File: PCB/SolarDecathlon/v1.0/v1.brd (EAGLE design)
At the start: 111.9 x 84.6 mm, 75 parts, among them CON1 SPI, IC1 REG1117, J1 RJ12, J2 RJ12, J3 RJ12, J4 RJ12, J5 RJ12, J6 RJ12, Q1 BSP75, Q2 BSP75, Q3 BSP75, Q4 BSP75, Q5 BSP75, Q6 BSP75, X3 16MHz, X4 MINI-USB

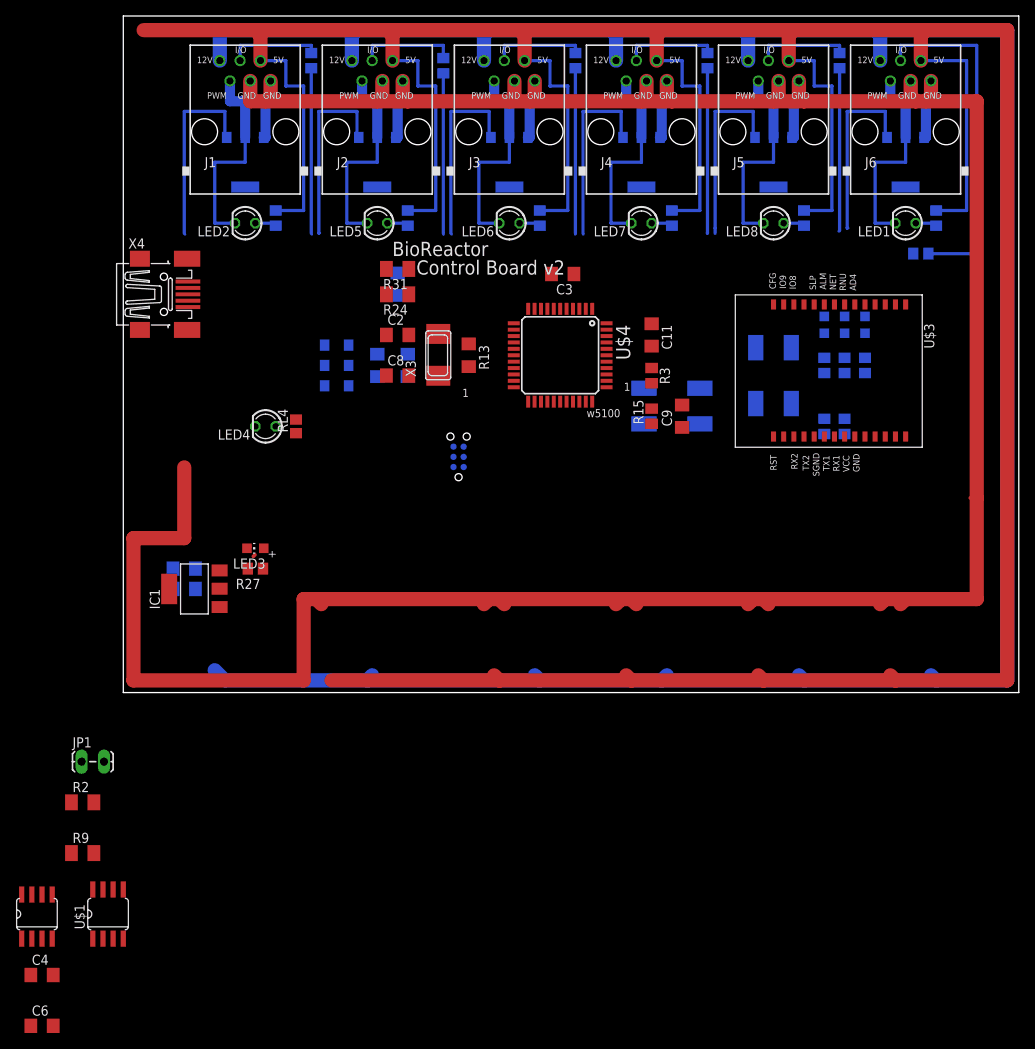
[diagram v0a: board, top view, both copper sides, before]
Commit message: Update wiegand
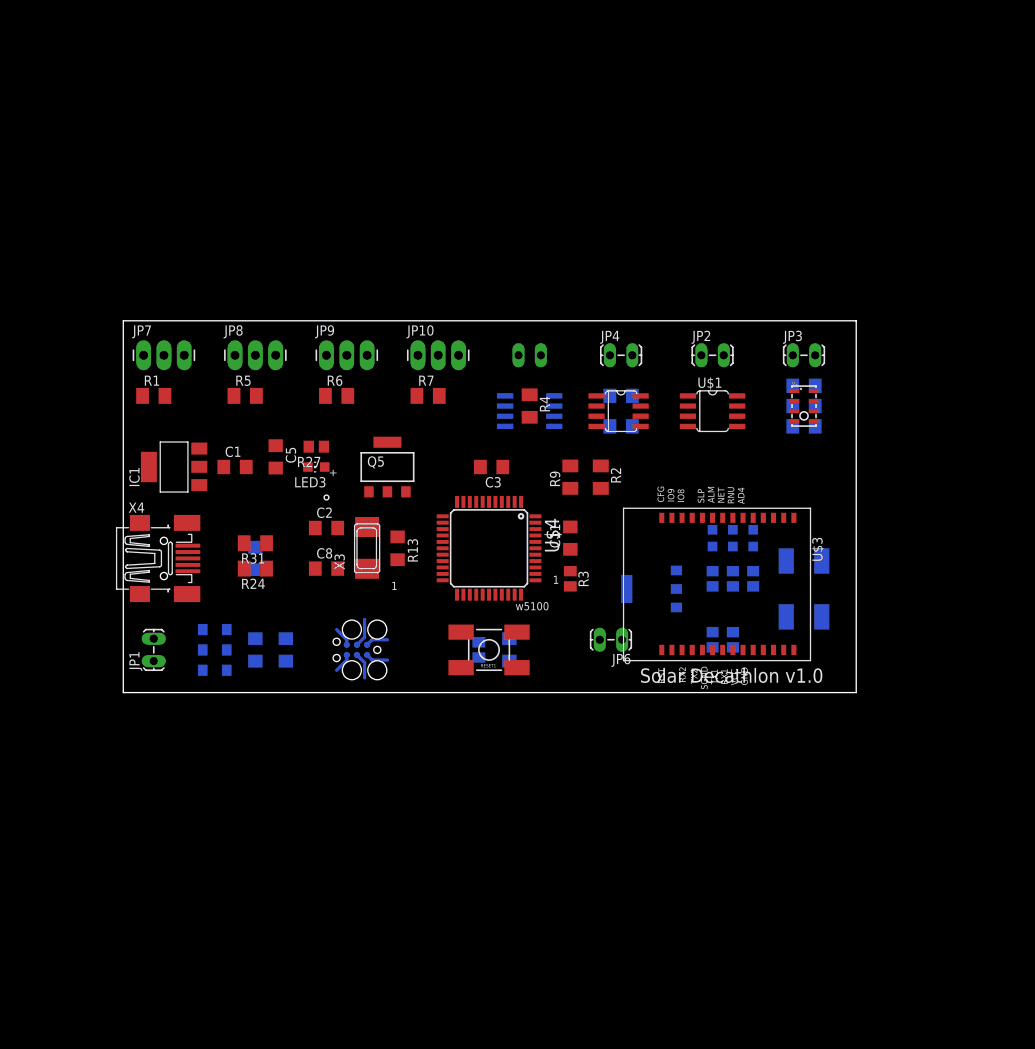
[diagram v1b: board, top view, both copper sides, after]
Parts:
- removed J1, J2, J3, J4, J5, J6: RJ12, lpatiny:RJ12-STRAIGHT
- removed LED1, LED2, LED5, LED6, LED8: Blue, lpatiny:LED3MM
- removed LED4: RED, lpatiny:LED3MM
- removed LED7: BLue, lpatiny:LED3MM
- removed Q1, Q2, Q4, Q6: BSP75, infineon:PG-SOT-223
- removed R, R19, R20, R25, R32, R33, R34, R35: 1k, rcl:R0805
- removed RL4: 1K, resistor:R0805
- added C13, C15: 100nF, rcl:C1206
- added C14: 10uF, rcl:C1206
- added JP10, JP7, JP8, JP9: (no value), SparkFun:1X03_LONGPADS
- added JP2, JP3, JP4, JP5, JP6: (no value), SparkFun:1X02_LOCK_LONGPADS
- added R1: 4.7k, resistor:M1206
- added U$5: DS18B20, lpatiny:SO8
- added U1: MPL3115A2LGA8, SparkFun-Sensors:LGA8
- CON1: device lpatiny:TC2030-MCP-NL -> lpatiny:TC2030-MCP
- R4, R5, R6, R7: value 1k -> 4.7k; device rcl:R0805 -> resistor:M1206
- moved C6 104.2 mm to (62.2, 30.5), flipped to the bottom, turned to 180 degrees
- moved C4 102.4 mm to (62.2, 34.3), flipped to the bottom, turned to 180 degrees
- moved U$1 95.6 mm to (73.7, 30.5), turned to 270 degrees
- moved U$2 95.5 mm to (62.2, 31.8), turned to 270 degrees
- moved R9 77.0 mm to (55.9, 24.1), turned to 90 degrees
- moved R2 76.5 mm to (59.7, 24.1), turned to 270 degrees
- moved Q3 62.1 mm to (66.0, 10.2), turned to 270 degrees
- moved R7 52.0 mm to (38.1, 34.3), flipped to the top, turned to 0 degrees
- moved Q5 49.6 mm to (33.0, 25.4), flipped to the top, turned to 0 degrees
- moved R6 47.4 mm to (26.7, 34.3), flipped to the top, turned to 0 degrees
- moved R5 43.0 mm to (15.2, 34.3), flipped to the top, turned to 0 degrees
- moved D2 41.0 mm to (11.4, 2.54)
- moved C10 38.7 mm to (16.5, 2.54)
- moved C12 38.7 mm to (20.3, 2.54)
- moved D3 38.7 mm to (11.4, 0.00)
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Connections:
- removed net +12V: J1.+12V, J2.+12V, J3.+12V, J4.+12V, J5.+12V, J6.+12V
- removed net N$1: J3.PWM, LED6.K, Q4.2
- removed net N$12: LED4.A, RL4.2
- removed net N$17: LED2.A, R25.1
- removed net N$18: J1.I/O, R.2
- removed net N$19: J5.PWM, LED8.K, Q6.2
- removed net N$21: J6.PWM, LED1.K, Q3.2
- removed net N$22: LED6.A, R5.1
- removed net N$28: J2.PWM, LED5.K, Q2.2
- removed net N$29: J4.I/O, R34.2
- removed net N$3: J6.I/O, R19.2
- removed net N$30: LED7.A, R6.1
- removed net N$32: J5.I/O, R35.2
- removed net N$33: LED8.A, R7.1
- removed net N$34: J1.PWM, LED2.K, Q1.2
- removed net N$4: LED5.A, R4.1
- removed net N$5: J4.PWM, LED7.K, Q5.2
- removed net N$7: J3.I/O, R33.2
- removed net N$9: LED1.A, R20.1
- new net $1: C13.2, C14.2, C15.2, JP3.1, U1.3
- new net $12: JP2.1, U$1.4
- new net $2: C4.2, C6.2, JP4.1, U$2.2
- new net $3: JP5.1, U$5.5
- new net GND_CONTROLLED: JP2.2, JP3.2, JP4.2, JP5.2, Q3.2, Q5.3
- new net N$13: C15.1, U1.2
- new net N$8: JP6.1, U$3.GND
- net +5V: no longer J1.+5V, J2.+5V, J3.+5V, J4.+5V, J5.+5V, J6.+5V, R20.2, R25.2, R4.2, R5.2, R6.2, R7.2
- net 3.3V: now also C13.1, C14.1, JP10.1, JP7.1, JP8.1, JP9.1, R1.1, R4.1, R5.1, R6.1, R7.1, U$5.3, U1.1, U1.4
- net A0: now also R4.2, U$5.4; no longer R35.1
- net A1: now also JP9.2, R6.2; no longer R33.1
- net A2: now also JP8.2, R5.2; no longer R32.1
- net A3: now also JP7.2, R1.2; no longer R.1
- net A4: now also JP10.2, R7.2; no longer R34.1
- net A5: no longer R19.1
- net D10*: no longer Q3.1
- net D11*: no longer Q6.1
- net D5*: no longer Q5.1
- net D6*: now also Q5.1; no longer Q1.1
- net D8*: now also Q3.1; no longer Q2.1
- net D9*: no longer Q4.1
- net GND: now also JP10.3, JP7.3, JP8.3, JP9.3; no longer C4.2, C6.2, J1.GND1, J1.GND2, J2.GND1, J2.GND2, J3.GND1, J3.GND2, J4.GND1, J4.GND2, J5.GND1, J5.GND2, J6.GND1, J6.GND2, LED4.K, Q1.3, Q2.3, Q4.3, Q5.3, Q6.3, U$1.4, U$2.2, U$3.GND
- net N$2: now also JP6.2, Q5.2; no longer J2.I/O, R32.2
- net SCL: now also U1.8
- net SDA: now also U1.7
- net VCC: no longer RL4.1
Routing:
- net +5V: track 468.1 -> 0.00 mm
- net GND: track 392.4 -> 2.43 mm
- net +12V: track 308.0 -> 0.00 mm
- net N$3: track 59.1 -> 0.00 mm
- net N$19: track 26.0 -> 0.00 mm
- net N$34: track 26.0 -> 0.00 mm
- net N$28: track 26.0 -> 0.00 mm
- net N$21: track 26.0 -> 0.00 mm
- net N$1: track 26.0 -> 0.00 mm
- net N$5: track 26.0 -> 0.00 mm
- net D6*: track 24.0 -> 0.00 mm
- net D9*: track 23.7 -> 0.00 mm
- net D5*: track 23.6 -> 0.00 mm
- net D8*: track 23.6 -> 0.00 mm
- net D11*: track 23.5 -> 0.00 mm
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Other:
- board size 111.9 x 84.6 mm -> 91.6 x 46.5 mm
- board text added: "Solar Decathlon v1.0"
- board text removed: "BioReactor"
- board text removed: "Control Board v2"

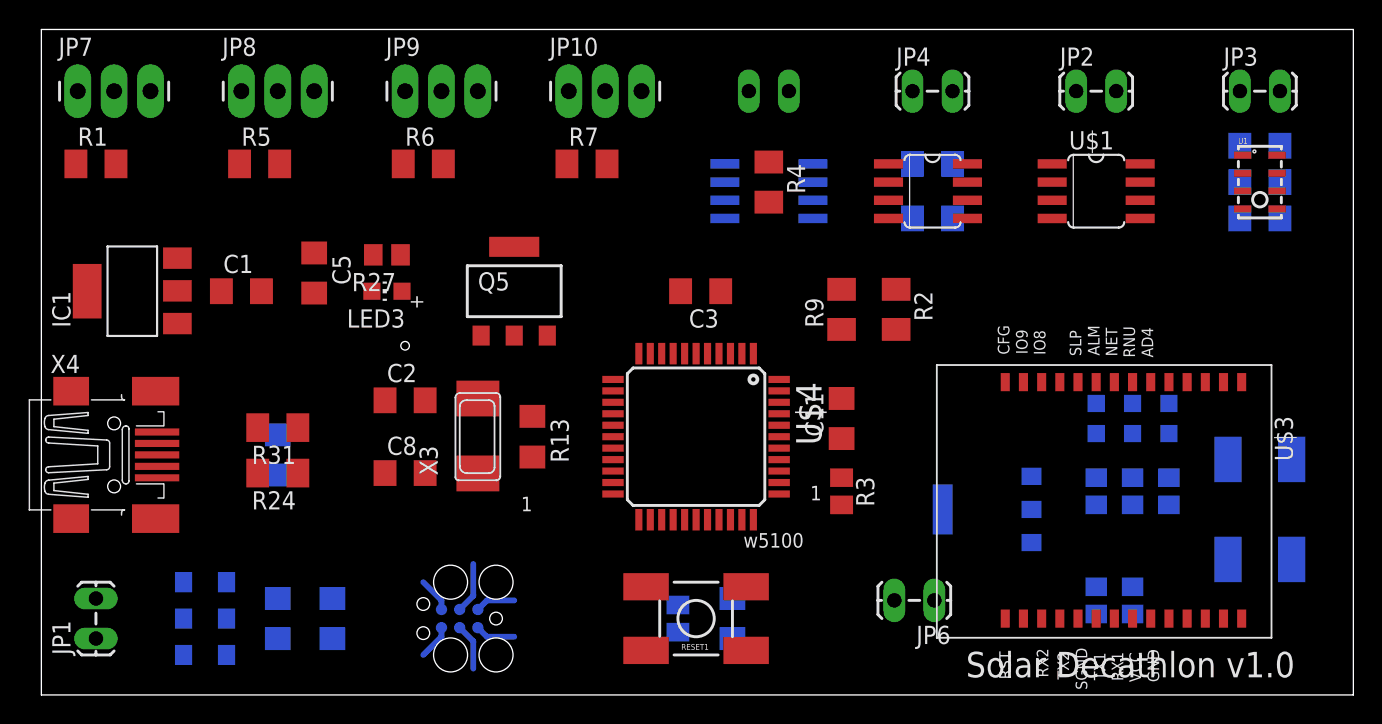
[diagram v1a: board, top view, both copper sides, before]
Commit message: Add routing
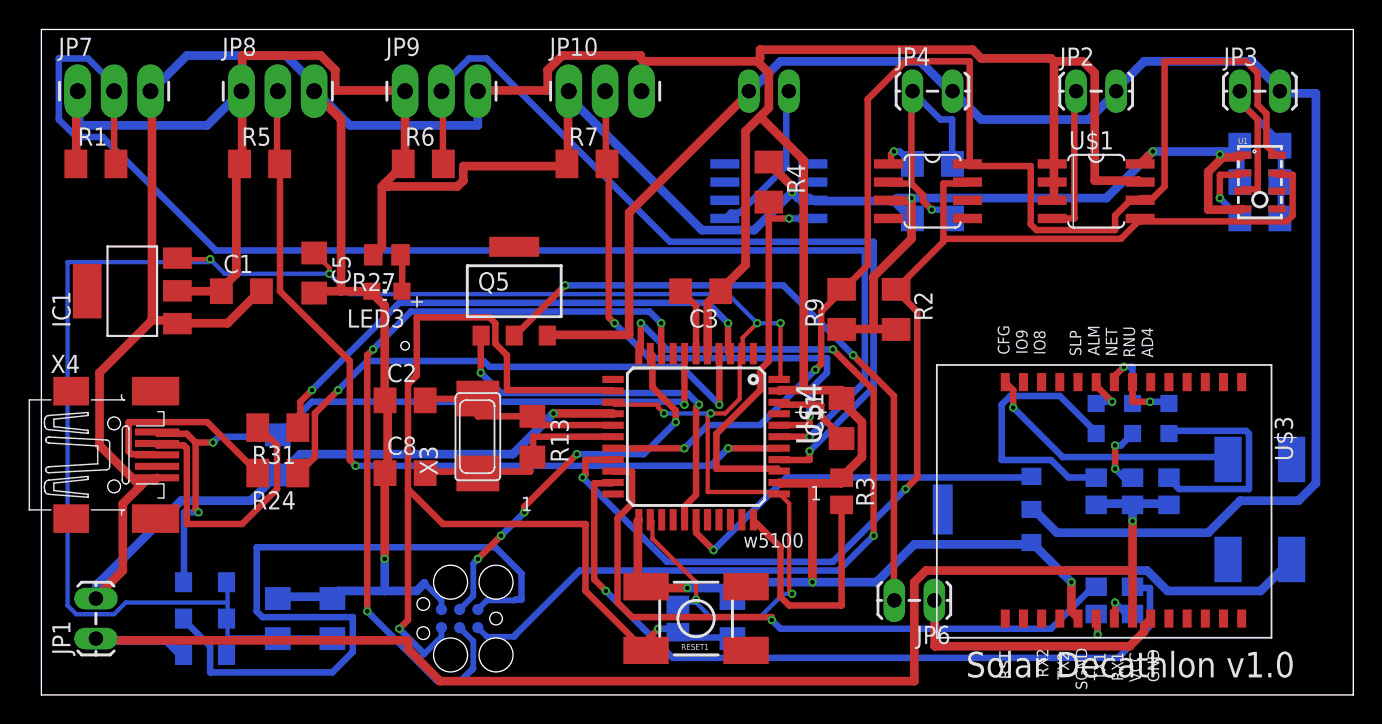
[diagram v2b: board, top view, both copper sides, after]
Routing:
- net GND: track 2.43 -> 368.3 mm, vias 0 -> 5
- net 3.3V: track 0.00 -> 171.5 mm, vias 0 -> 4
- net VCC: track 0.00 -> 158.4 mm, vias 0 -> 8
- net GND_CONTROLLED: track 0.00 -> 120.3 mm
- net +5V: track 0.00 -> 101.0 mm, vias 0 -> 1
- net SCL: track 0.00 -> 94.2 mm, vias 0 -> 2
- net A3: track 0.00 -> 91.3 mm, vias 0 -> 1
- net SDA: track 0.00 -> 85.1 mm, vias 0 -> 2
- net RESET: track 2.43 -> 76.7 mm, vias 0 -> 2
- net A1: track 0.00 -> 61.0 mm, vias 0 -> 1
- net MISO: track 2.80 -> 61.4 mm, vias 0 -> 3
- net A2: track 0.00 -> 58.6 mm, vias 0 -> 2
- net TX: track 0.00 -> 54.0 mm, vias 0 -> 1
- net VUSB: track 0.00 -> 52.9 mm, vias 0 -> 3
- net SCK: track 3.25 -> 55.2 mm, vias 0 -> 3
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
